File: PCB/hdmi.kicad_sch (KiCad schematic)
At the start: 22 parts, among them J3 HDMI-019S, U12 PCA9306DC1

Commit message: basic HDMI ESD protection I think
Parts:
- added U14, U15, U16: ESD224DQAR-TP, Package_DFN_QFN:Diodes_UDFN-10_1.0x2.5mm_P0.5mm, symbol Power_Protection:ESD224DQA
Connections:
- net GND: now also U14.3 (VSS), U14.8 (VSS), U15.3 (VSS), U15.8 (VSS), U16.3 (VSS), U16.8 (VSS)
- net HDMI_CEC: now also U16.1, U16.10
- net HDMI_CLK+: now also U15.4, U15.7
- net HDMI_CLK-: now also U15.5, U15.6
- net HDMI_D0+: now also U15.1, U15.10
- net HDMI_D0-: now also U15.2, U15.9
- net HDMI_D1+: now also U14.4, U14.7
- net HDMI_D1-: now also U14.5, U14.6
- net HDMI_D2+: now also U14.1, U14.10
- net HDMI_D2-: now also U14.2, U14.9
- net HDMI_HPD: now also U16.2, U16.9
- net HDMI_SCL: now also U16.4, U16.7
- net HDMI_SDA: now also U16.5, U16.6
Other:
- note added: "5V vs 3.6V?"
- note removed: "DOUBLE CHECK AC CAPS, ESD PROTECTION"
- moved on the sheet: C113, C114, C115, C116, C117, C119, C120, C121, C122, C123, C14, C16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

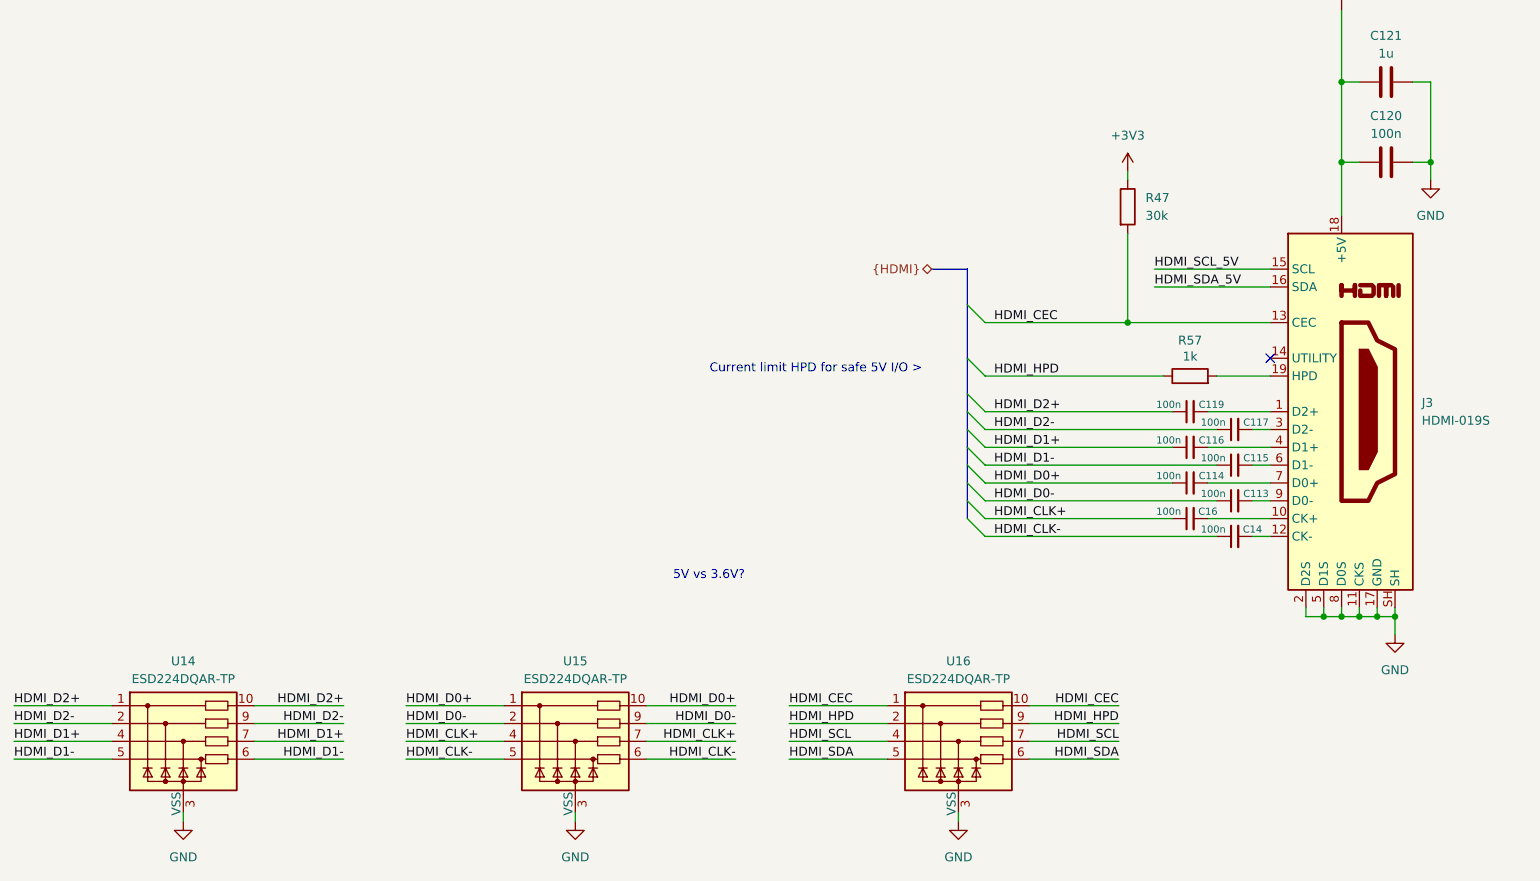
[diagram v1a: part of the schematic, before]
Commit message: finished HDMI ESD protection, took longer than I would have liked
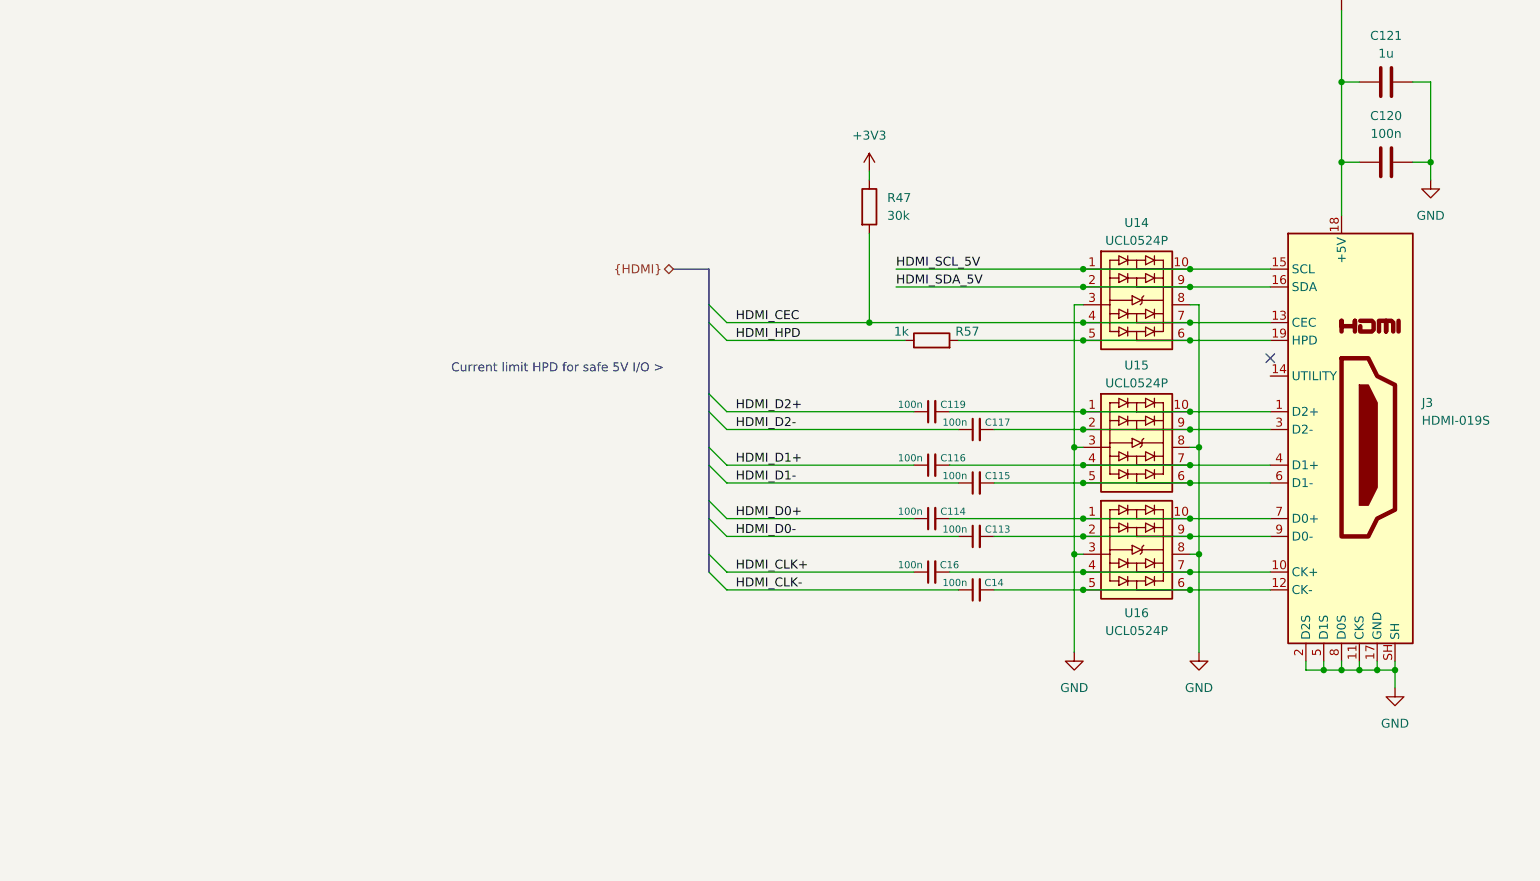
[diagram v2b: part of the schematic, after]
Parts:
- removed U14, U15, U16: ESD224DQAR-TP, Package_DFN_QFN:Diodes_UDFN-10_1.0x2.5mm_P0.5mm, symbol Power_Protection:ESD224DQA
- added U14, U15, U16: UCL0524P, Package_DFN_QFN:Diodes_UDFN-10_1.0x2.5mm_P0.5mm, symbol kai-library:UCL0524P
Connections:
- net GND: now also U14.3, U14.8, U15.3, U15.8, U16.3, U16.8
- net HDMI_CEC: now also U14.4, U14.7
- net HDMI_SCL_5V: now also U14.1, U14.10
- net HDMI_SDA_5V: now also U14.2, U14.9
- net at J3.19 (HPD), R57.2: now also U14.5, U14.6
- net at C117.2, J3.3 (D2-): now also U15.2, U15.9
- net at C116.2, J3.4 (D1+): now also U15.4, U15.7
- net at C114.2, J3.7 (D0+): now also U16.1, U16.10
- net at C119.2, J3.1 (D2+): now also U15.1, U15.10
- net at C16.2, J3.10 (CK+): now also U16.4, U16.7
- net at C14.2, J3.12 (CK-): now also U16.5, U16.6
- net at C115.2, J3.6 (D1-): now also U15.5, U15.6
- net at C113.2, J3.9 (D0-): now also U16.2, U16.9
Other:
- note removed: "5V vs 3.6V?"
- moved on the sheet: C113, C114, C115, C116, C117, C119, C14, C16, J3, R47, R57
